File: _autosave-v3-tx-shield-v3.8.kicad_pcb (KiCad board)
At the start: 2 copper layers, 116.8 x 58.4 mm, 109 parts, among them J1 Conn_01x08_Male, J2 Conn_01x02_Male, J3 Conn_01x02_Male, P1 Power, P2 Analog, P3 Digital, P4 Digital

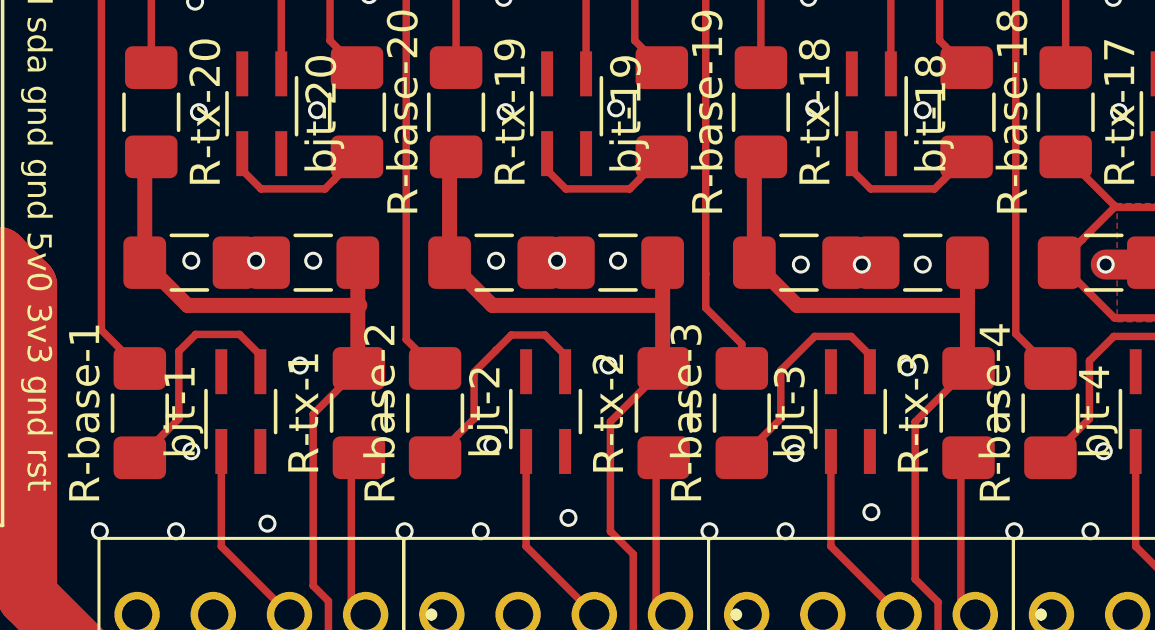
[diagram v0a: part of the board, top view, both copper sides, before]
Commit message: Final version
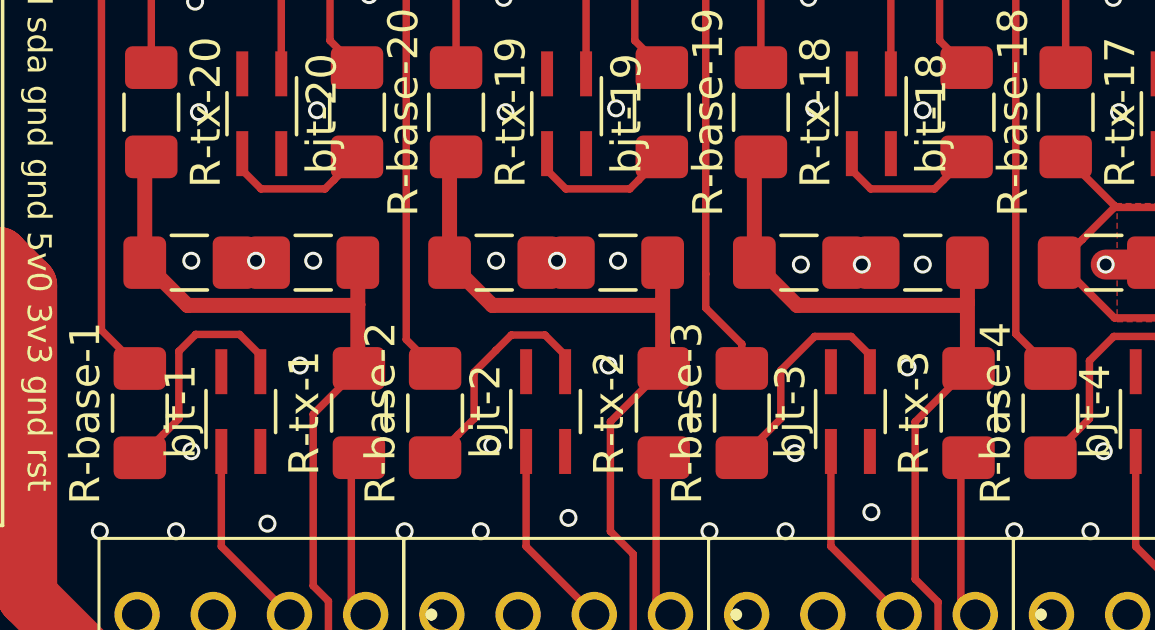
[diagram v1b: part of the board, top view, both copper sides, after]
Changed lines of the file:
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@@
     (thickness 1.6)
     (drawings 50)
-    (tracks 658)
+    (tracks 659)
     (zones 0)
     (modules 109)
@@
   )
   (layers
-    (0 F.Cu signal)
-    (31 B.Cu signal)
-    (32 B.Adhes user)
-    (33 F.Adhes user)
+    (0 F.Cu signal hide)
+    (31 B.Cu signal hide)
+    (32 B.Adhes user hide)
+    (33 F.Adhes user hide)
     (34 B.Paste user hide)
-    (35 F.Paste user)
-    (36 B.SilkS user)
-    (37 F.SilkS user)
+    (35 F.Paste user hide)
+    (36 B.SilkS user hide)
+    (37 F.SilkS user hide)
     (38 B.Mask user hide)
     (39 F.Mask user hide)
@@
   (segment (start 146.94001 101.05651) (end 152.58949 101.05651) (width 0.5) (layer F.Cu) (net 3))
   (segment (start 145.515 99.6315) (end 146.94001 101.05651) (width 0.5) (layer F.Cu) (net 3))
-  (segment (start 136.78001 101.05651) (end 142.52949 101.05651) (width 0.5) (layer F.Cu) (net 3))
   (segment (start 135.355 99.6315) (end 136.78001 101.05651) (width 0.5) (layer F.Cu) (net 3))
   (segment (start 142.4575 103.12146) (end 142.494 103.15796) (width 0.5) (layer F.Cu) (net 3))
-  (segment (start 142.4575 99.6315) (end 142.4575 103.12146) (width 0.5) (layer F.Cu) (net 3))
   (segment (start 152.6175 103.12146) (end 152.654 103.15796) (width 0.5) (layer F.Cu) (net 3))
   (segment (start 152.6175 99.6315) (end 152.6175 103.12146) (width 0.5) (layer F.Cu) (net 3))
   (segment (start 162.7775 103.12146) (end 162.814 103.15796) (width 0.5) (layer F.Cu) (net 3))
-  (segment (start 162.68599 101.05651) (end 162.7775 100.965) (width 0.5) (layer F.Cu) (net 3))
   (segment (start 157.10001 101.05651) (end 162.68599 101.05651) (width 0.5) (layer F.Cu) (net 3))
   (segment (start 155.675 99.6315) (end 157.10001 101.05651) (width 0.5) (layer F.Cu) (net 3))
@@
   (segment (start 155.675 96.32254) (end 155.8925 96.10504) (width 0.5) (layer F.Cu) (net 3))
   (segment (start 155.675 99.6315) (end 155.675 96.32254) (width 0.5) (layer F.Cu) (net 3))
+  (segment (start 142.42949 101.05651) (end 142.4575 101.0285) (width 0.5) (layer F.Cu) (net 3))
+  (segment (start 136.78001 101.05651) (end 142.42949 101.05651) (width 0.5) (layer F.Cu) (net 3))
+  (segment (start 142.4575 99.6315) (end 142.4575 101.0285) (width 0.5) (layer F.Cu) (net 3))
+  (segment (start 142.4575 101.0285) (end 142.4575 103.12146) (width 0.5) (layer F.Cu) (net 3))
   (via (at 139.065 99.568) (size 0.6) (drill 0.4) (layers F.Cu B.Cu) (net 4))
   (via (at 149.098 99.568) (size 0.6) (drill 0.4) (layers F.Cu B.Cu) (net 4))
